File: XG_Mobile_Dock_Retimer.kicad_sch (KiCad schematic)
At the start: 248 parts, among them J1 5-1775443-8, J13 39301240, J14 469911008, J17 8730, J2 20455-040E-76, J3 20455-040E-76, J7 CEE016400140111, SW1 SW_Push, U1 DS160PT801ACBR, U2 TPS7A8400ARGRR, U7 TPS7A8400ARGRR

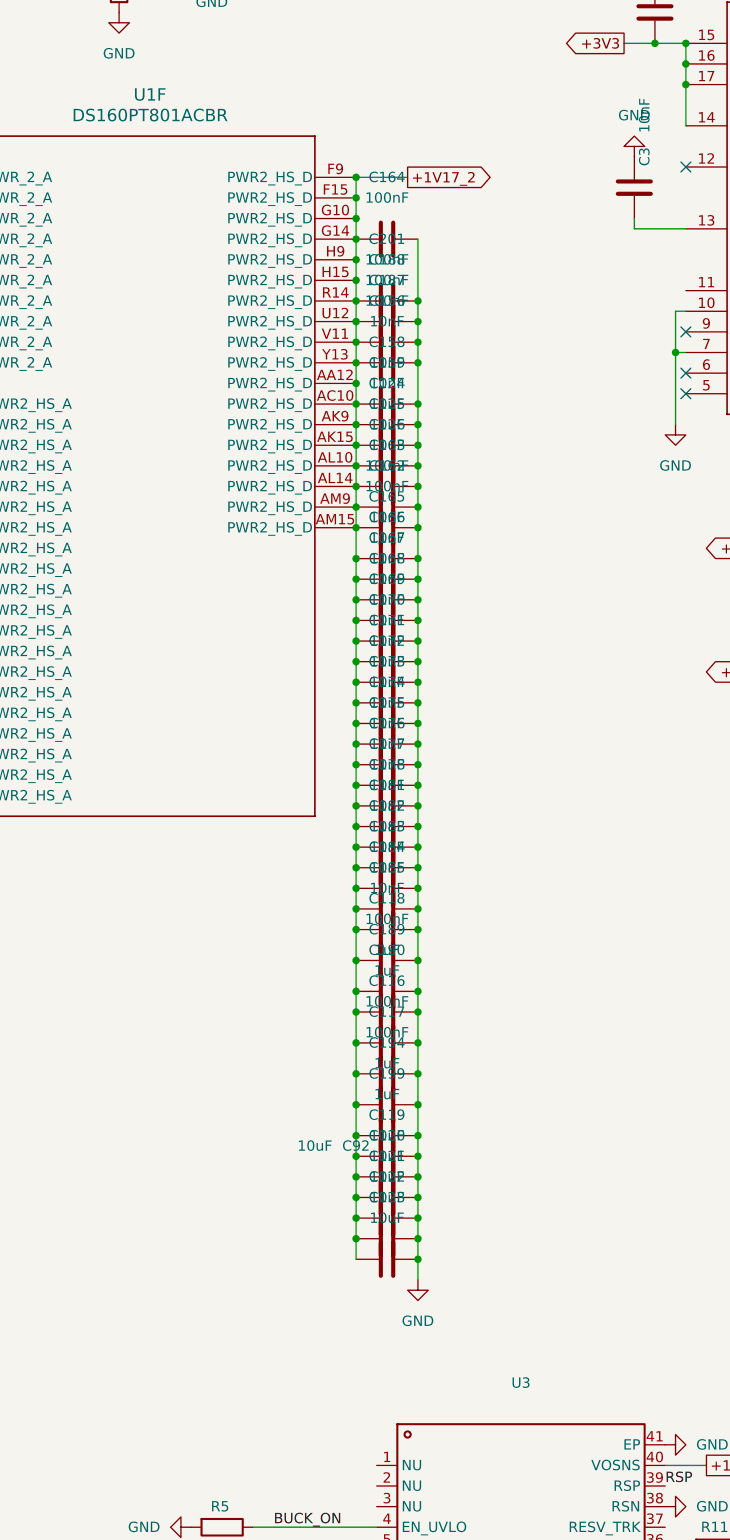
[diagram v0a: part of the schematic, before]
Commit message: eee
eee
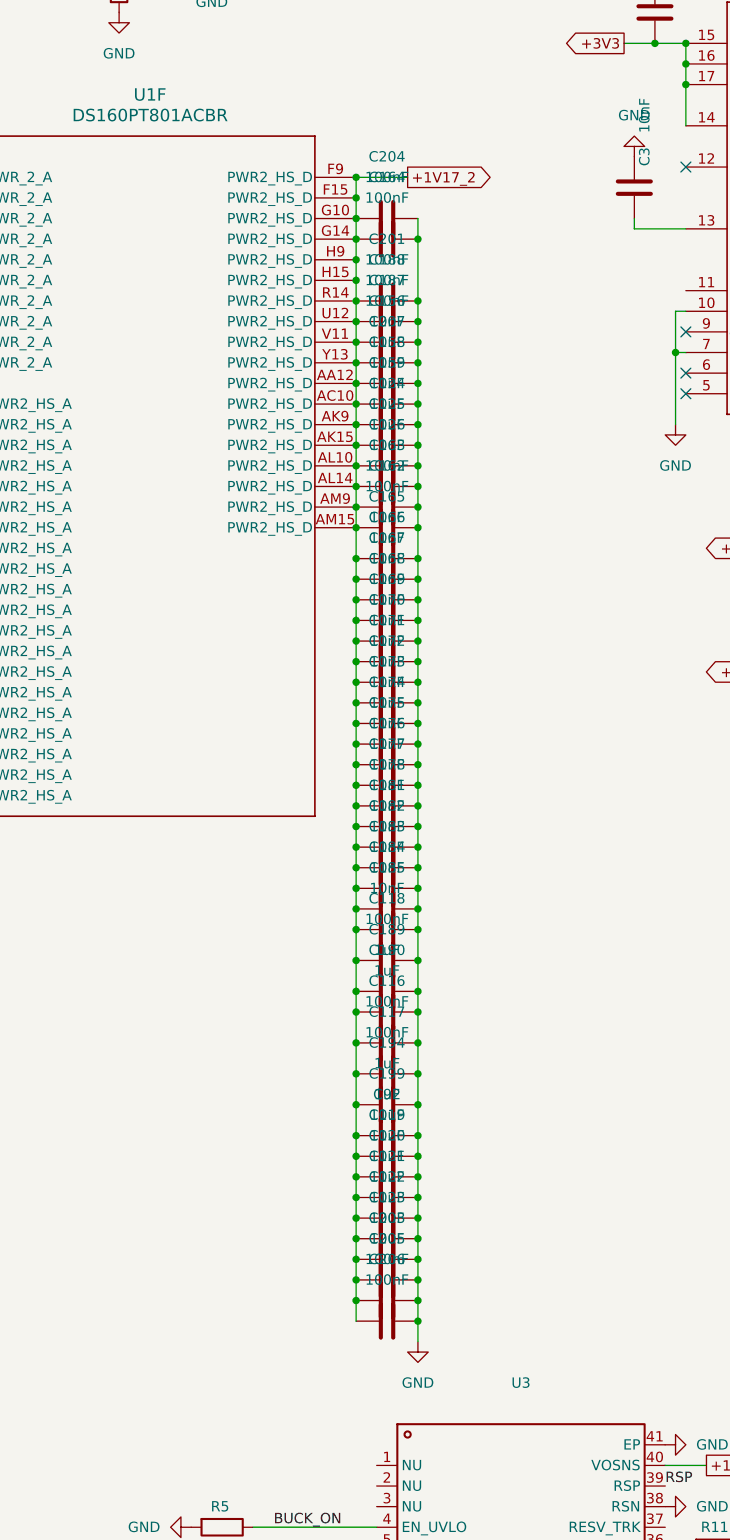
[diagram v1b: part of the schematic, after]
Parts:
- added C203, C207: 10uF, Capacitor_SMD:C_0402_1005Metric, symbol Device:C
- added C204, C205, C206: 100nF, Capacitor_SMD:C_0201_0603Metric, symbol Device:C
- C92: footprint Capacitor_SMD:C_0805_2012Metric -> Capacitor_SMD:C_0402_1005Metric; LCSC C15850 -> C15525; Part_Number CL21A106KAYNNNE -> CL05A106MQ5NUNC
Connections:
- net +1V17_2: now also C92.2, C203.2, C204.2, C205.2, C206.2, C207.2; no longer C92.1
- net GND: now also C92.1, C203.1, C204.1, C205.1, C206.1, C207.1; no longer C92.2
